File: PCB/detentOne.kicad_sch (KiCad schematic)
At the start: 9 parts, among them J5 Conn_01x05, SW7 C92589, SW8 C92589, U1 ESP32-S3-WROOM-1U-N16R8

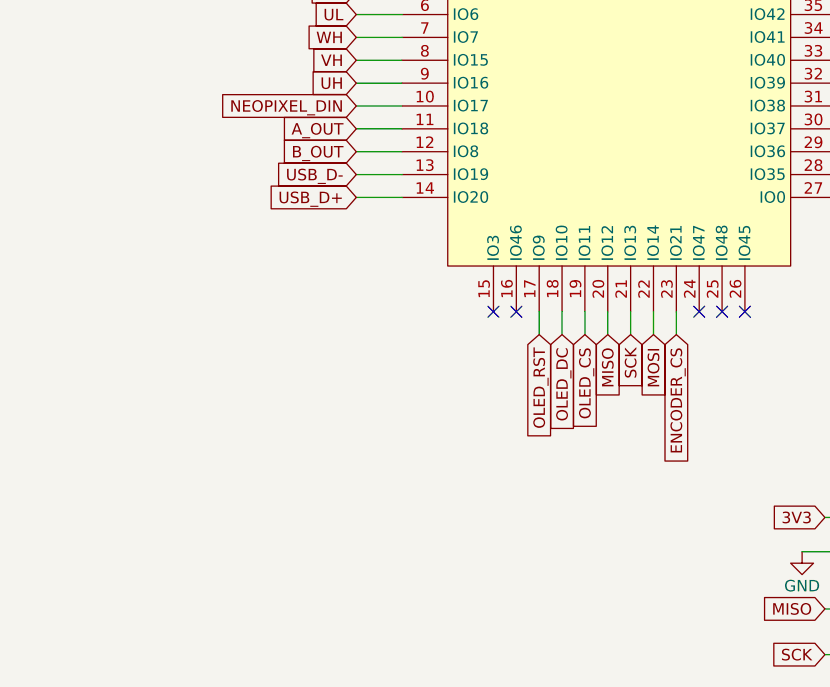
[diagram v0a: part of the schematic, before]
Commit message: final checks for PCB, nearly ready to order v1
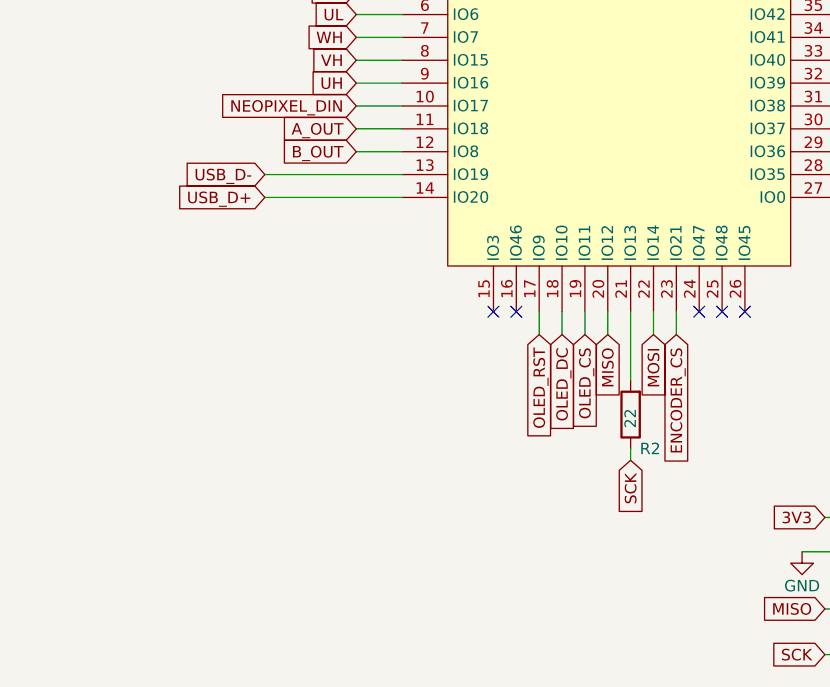
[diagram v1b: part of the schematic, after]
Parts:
- added R2: 22, Resistor_SMD:R_0402_1005Metric_Pad0.72x0.64mm_HandSolder, symbol Device:R
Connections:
- net SCK: now also R2.1; no longer U1.21 (IO13)
- new net: R2.2, U1.21 (IO13)
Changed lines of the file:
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@@
 	(wire
 		(pts
-			(xy 210.82 110.49) (xy 210.82 113.03)
-		)
-		(stroke
-			(width 0)
-			(type default)
-		)
-	)
-	(wire
-		(pts
 			(xy 236.22 148.59) (xy 236.22 146.05)
 		)
@@
 	(wire
 		(pts
+			(xy 210.82 110.49) (xy 210.82 118.11)
+		)
+		(stroke
+			(width 0)
+			(type default)
+		)
+	)
+	(wire
+		(pts
 			(xy 213.36 110.49) (xy 213.36 113.03)
 		)
@@
 	(wire
 		(pts
-			(xy 180.34 97.79) (xy 185.42 97.79)
+			(xy 170.18 97.79) (xy 185.42 97.79)
 		)
 		(stroke
@@
 	(wire
 		(pts
-			(xy 180.34 95.25) (xy 185.42 95.25)
+			(xy 210.82 125.73) (xy 210.82 127)
+		)
+		(stroke
+			(width 0)
+			(type default)
+		)
+	)
+	(wire
+		(pts
+			(xy 170.18 95.25) (xy 185.42 95.25)
 		)
 		(stroke
@@
 	(global_label "USB_D-"
 		(shape input)
-		(at 180.34 95.25 180)
+		(at 170.18 95.25 180)
 		(fields_autoplaced yes)
 		(effects
@@
 		)
 		(property "Intersheetrefs" "${INTERSHEET_REFS}"
-			(at 169.7348 95.25 0)
+			(at 159.5748 95.25 0)
 			(effects
 				(font
@@
 	(global_label "USB_D+"
 		(shape input)
-		(at 180.34 97.79 180)
+		(at 170.18 97.79 180)
 		(fields_autoplaced yes)
 		(effects
@@
 		)
 		(property "Intersheetrefs" "${INTERSHEET_REFS}"
-			(at 169.7348 97.79 0)
+			(at 159.5748 97.79 0)
 			(effects
 				(font
@@
 	(global_label "SCK"
 		(shape input)
-		(at 210.82 113.03 270)
+		(at 210.82 127 270)
 		(fields_autoplaced yes)
 		(effects
@@
 		)
 		(property "Intersheetrefs" "${INTERSHEET_REFS}"
-			(at 210.82 119.7647 90)
+			(at 210.82 133.7347 90)
 			(effects
 				(font
@@
 					(unit 1)
 				)
+			)
+		)
+	)
+	(symbol
+		(lib_id "Device:R")
+		(at 210.82 121.92 180)
+		(unit 1)
+		(exclude_from_sim no)
+		(in_bom yes)
+		(on_board yes)
+		(dnp no)
+		(property "Reference" "R2"
+			(at 211.836 125.73 0)
+			(effects
+				(font
+					(size 1.27 1.27)
+				)
+				(justify right)
+			)
+		)
+		(property "Value" "22"
+			(at 210.82 123.444 90)
+			(effects
+				(font
+					(size 1.27 1.27)
+				)
+				(justify right)
+			)
+		)
+		(property "Footprint" "Resistor_SMD:R_0402_1005Metric_Pad0.72x0.64mm_HandSolder"
+			(at 212.598 121.92 90)
+			(effects
+				(font
+					(size 1.27 1.27)
+				)
+				(hide yes)
+			)
+		)
+		(property "Datasheet" "~"
+			(at 210.82 121.92 0)
+			(effects
+				(font
+					(size 1.27 1.27)
+				)
+				(hide yes)
+			)
+		)
+		(property "Description" "Resistor"
+			(at 210.82 121.92 0)
+			(effects
+				(font
+					(size 1.27 1.27)
+				)
+				(hide yes)
+			)
+		)
+		(property "Sim.Device" ""
+			(at 210.82 121.92 0)
+			(effects
+				(font
+					(size 1.27 1.27)
+				)
+			)
+		)
+		(property "Sim.Type" ""
+			(at 210.82 121.92 0)
+			(effects
+				(font
+					(size 1.27 1.27)
+				)
+			)
+		)
+		(pin "2"
+		)
+		(pin "1"
+		)
+		(instances
+			(project "detentOne"
+				(path "/64c66767-4367-4391-b4db-5d3ae338f23b"
+					(reference "R2")
+					(unit 1)
+				)
